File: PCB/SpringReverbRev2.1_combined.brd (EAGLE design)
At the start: 107 x 60.8 mm, 87 parts, among them IC102 TL074, IC103 TL074, J1 MA08-1, J2 MA08-1, U1 TL072_, U2 TL072_, U7 NE5532

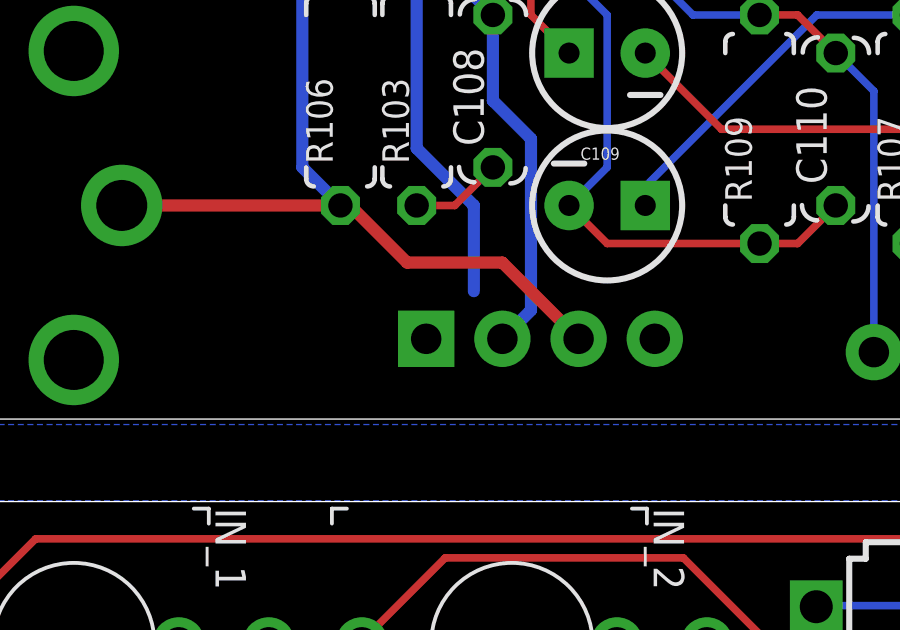
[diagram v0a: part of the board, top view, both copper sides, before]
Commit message: Fixes #18
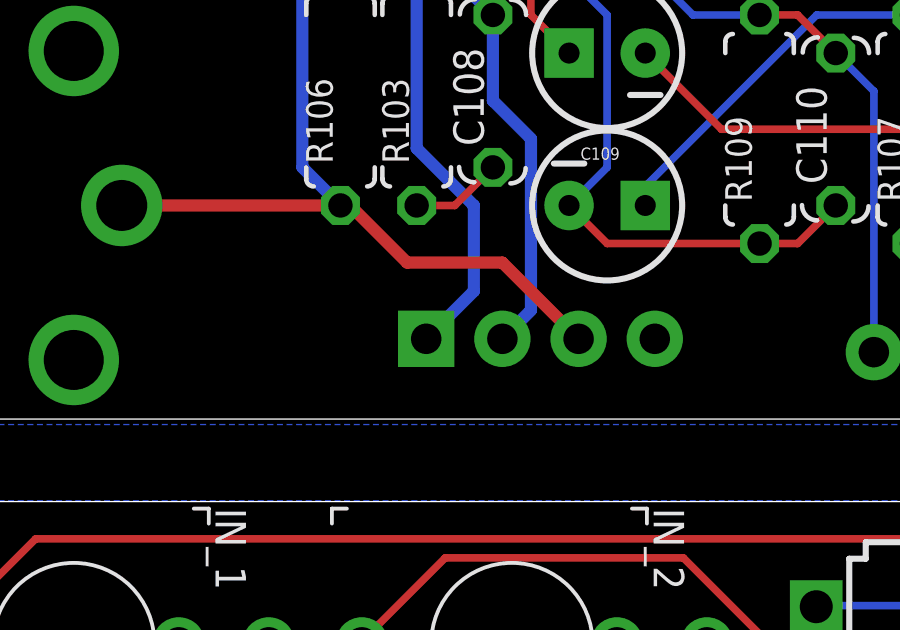
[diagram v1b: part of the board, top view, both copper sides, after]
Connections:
- removed net N$14: JP101.1
- net S+: now also JP101.1
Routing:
- net S+: track 44.6 -> 46.9 mm
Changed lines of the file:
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@@
 <wire x1="17.78" y1="46.99" x2="16.58" y2="48.19" width="0.4064" layer="1"/>
 <wire x1="16.58" y1="48.19" x2="6.35" y2="48.19" width="0.4064" layer="1"/>
+<contactref element="JP101" pad="1"/>
+<wire x1="19.685" y1="36.5125" x2="18.0975" y2="34.925" width="0.4064" layer="16"/>
 </signal>
 <signal name="N$26">
@@
 <wire x1="73.66" y1="2.2225" x2="74.93" y2="0.9525" width="0.254" layer="16"/>
 </signal>
-<signal name="N$14">
-<contactref element="JP101" pad="1"/>
-</signal>
 </signals>
